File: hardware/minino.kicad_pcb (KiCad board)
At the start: 2 copper layers, 42 x 68 mm, 52 parts, among them J1 OLED, J2 GPS, J3 Battery, P1 USB_C_Plug_USB2.0, Q1 DMG3415U-7, Q2 PN2222A, SW1 ON, SW2 RIGHT, SW3 LEFT, SW4 DOWN, SW5 UP, SW6 OK, SW7 RESET, SW8 GPIO, U1 ESP32-S3-WROOM-1U-N16, U2 MCP73831-3-OT, U3 AP2112K-3.3

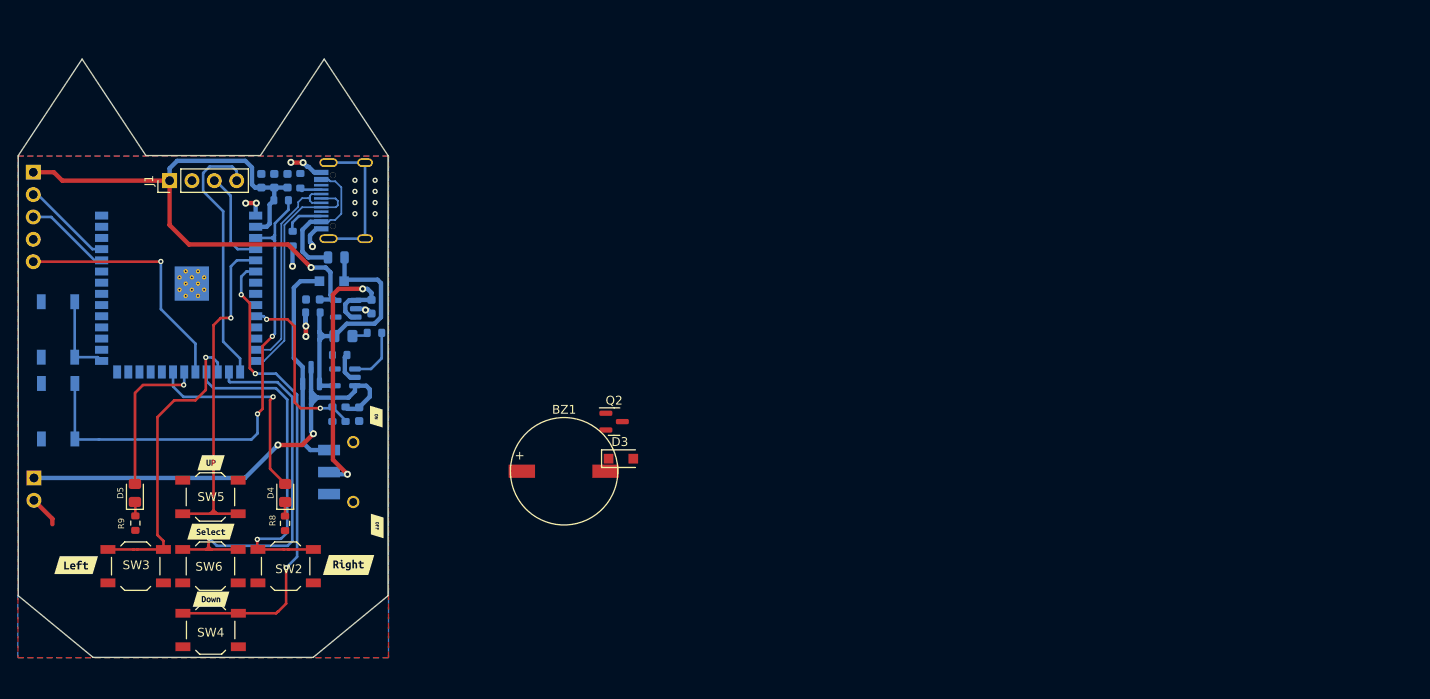
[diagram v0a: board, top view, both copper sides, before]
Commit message: Update_design
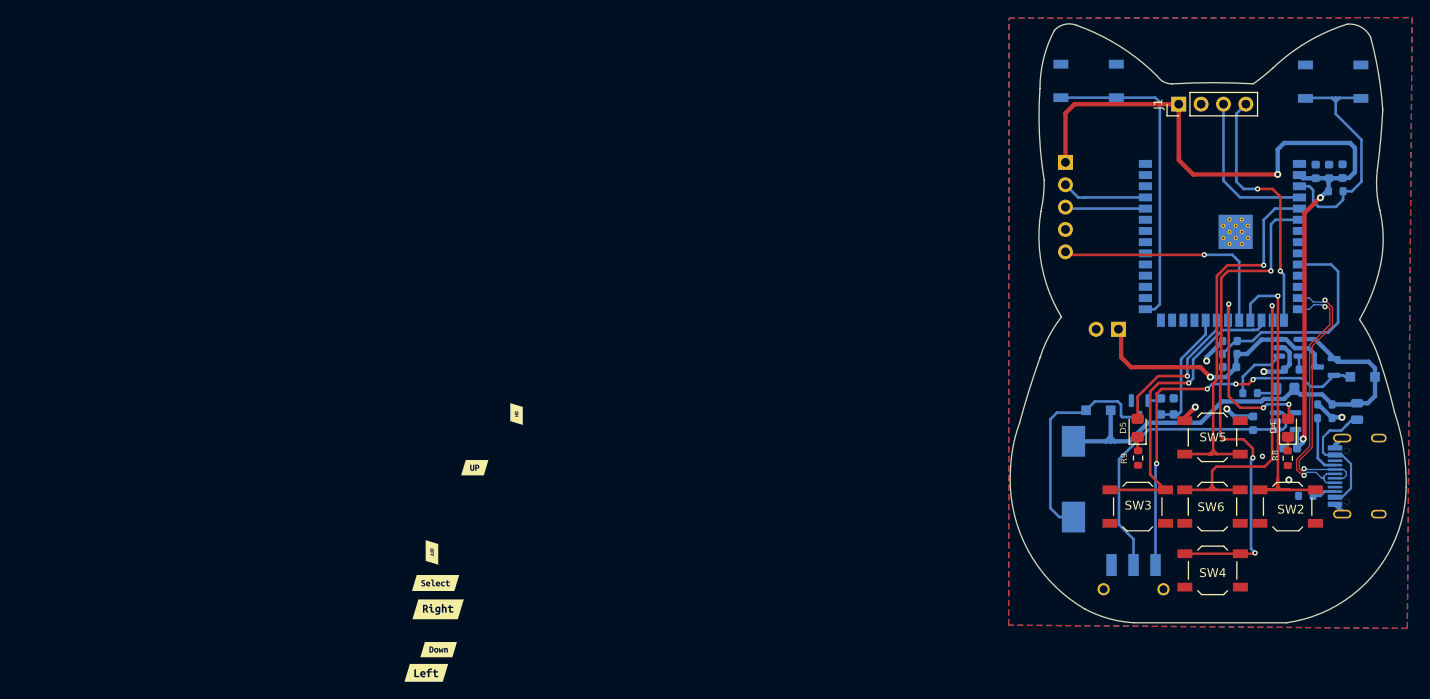
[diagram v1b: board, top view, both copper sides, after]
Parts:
- added R6: 1.1K, Resistor_SMD:R_0603_1608Metric_Pad0.98x0.95mm_HandSolder, B.Cu at (180.8, 75.5)
- added R7: 10K, Resistor_SMD:R_0603_1608Metric_Pad0.98x0.95mm_HandSolder, B.Cu at (182.2, 75.5)
- added Ref**: Val**, Aesthetics:01.PCB, F.Cu at (257.7, 152.6)
- BZ1: footprint Buzzer_Beeper:MagneticBuzzer_ProSignal_ABI-009-RC -> Footprint:CAPAE1050X250N; moved to B.Cu
- D3, Q2: moved to B.Cu
- moved SW7 149.6 mm to (200.4, 38.6), turned to 180 degrees
- moved J3 124.3 mm to (176.0, 66.7), turned to 90 degrees
- moved kibuzzard-6397B251 120.8 mm to (176.4, 70.2), turned to -90 degrees
- moved SW8 120.4 mm to (172.6, 38.5), turned to 180 degrees
- moved C3 119.8 mm to (201.4, 48.8)
- moved C2 119.8 mm to (199.9, 48.8)
- moved R12 119.8 mm to (200.7, 51.1)
- moved C4 119.8 mm to (198.4, 48.8)
- moved R10 119.5 mm to (199.4, 76.8), turned to 180 degrees
- moved P1 119.3 mm to (201.4, 83.4)
- moved R11 118.7 mm to (197.2, 85.7), turned to 0 degrees
- moved U1 118.7 mm to (187.8, 56.4)
- moved kibuzzard-6397B263 118.0 mm to (173.1, 70.3), turned to -90 degrees
- moved D2 117.6 mm to (203.7, 72.1)
- moved F1 117.3 mm to (203.1, 76.1), turned to 90 degrees
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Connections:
- J2 pad 5: /D1 -> /DIO11
- P1 pad S1: unconnected-(P1-PadS1) -> GND
- U1 pad 20: /LED1 -> /LED2
- U1 pad 21: /LED2 -> /LED1
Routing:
- net /RST: track 58.1 -> 28.9 mm, vias 2 -> 0
- net /D1: track 28.7 -> 0.00 mm, vias 1 -> 0
- net /DIO11: track 0.00 -> 26.9 mm, vias 0 -> 1
- net /BOOT: track 9.53 -> 36.3 mm
- net VBUS: track 29.7 -> 56.1 mm
- net Net-(BZ1-Pad2): track 0.00 -> 25.6 mm
- net +BATT: track 55.5 -> 31.1 mm, vias 2 -> 1
- net +3V3: track 70.3 -> 93.5 mm, vias 1 -> 3
- net Net-(D2-Pad1): track 24.6 -> 43.3 mm, vias 0 -> 4
- net unconnected-(P1-PadS1): track 16.9 -> 0.00 mm
- net /Buzz: track 0.00 -> 14.0 mm
- net /SELECT: track 44.0 -> 36.6 mm
- net /SCL: track 11.0 -> 18.1 mm
- net /D-: track 25.1 -> 31.7 mm, vias 0 -> 2
- net /B_ADC: track 20.4 -> 25.6 mm, vias 2 -> 0
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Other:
- board size 42 x 68 mm -> 45 x 68 mm
